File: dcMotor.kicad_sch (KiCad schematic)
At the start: 114 parts, among them J1 USB_C_Receptacle_USB2.0_16P, J2 USB_C_Receptacle_USB2.0_16P, J3 Conn_ST_STDC14, J6 Conn_01x02_Pin, J7 Conn_01x04_Pin, J8 Conn_01x06_Pin, Q1 AO3400A, SW1 SW_Push, SW2 SW_Push, U1 LMR54406DBVR, U10 MCP6561-OT, U2 NCP718ASNADJT1G, U3 NCP718ASNADJT1G, U5 TLV9152IDR, U6 ER_OLEDM0.91_1x-I2C, U7 STM32G431CBTx, U8 LTH-301-05, U9 DRV8231ADDA

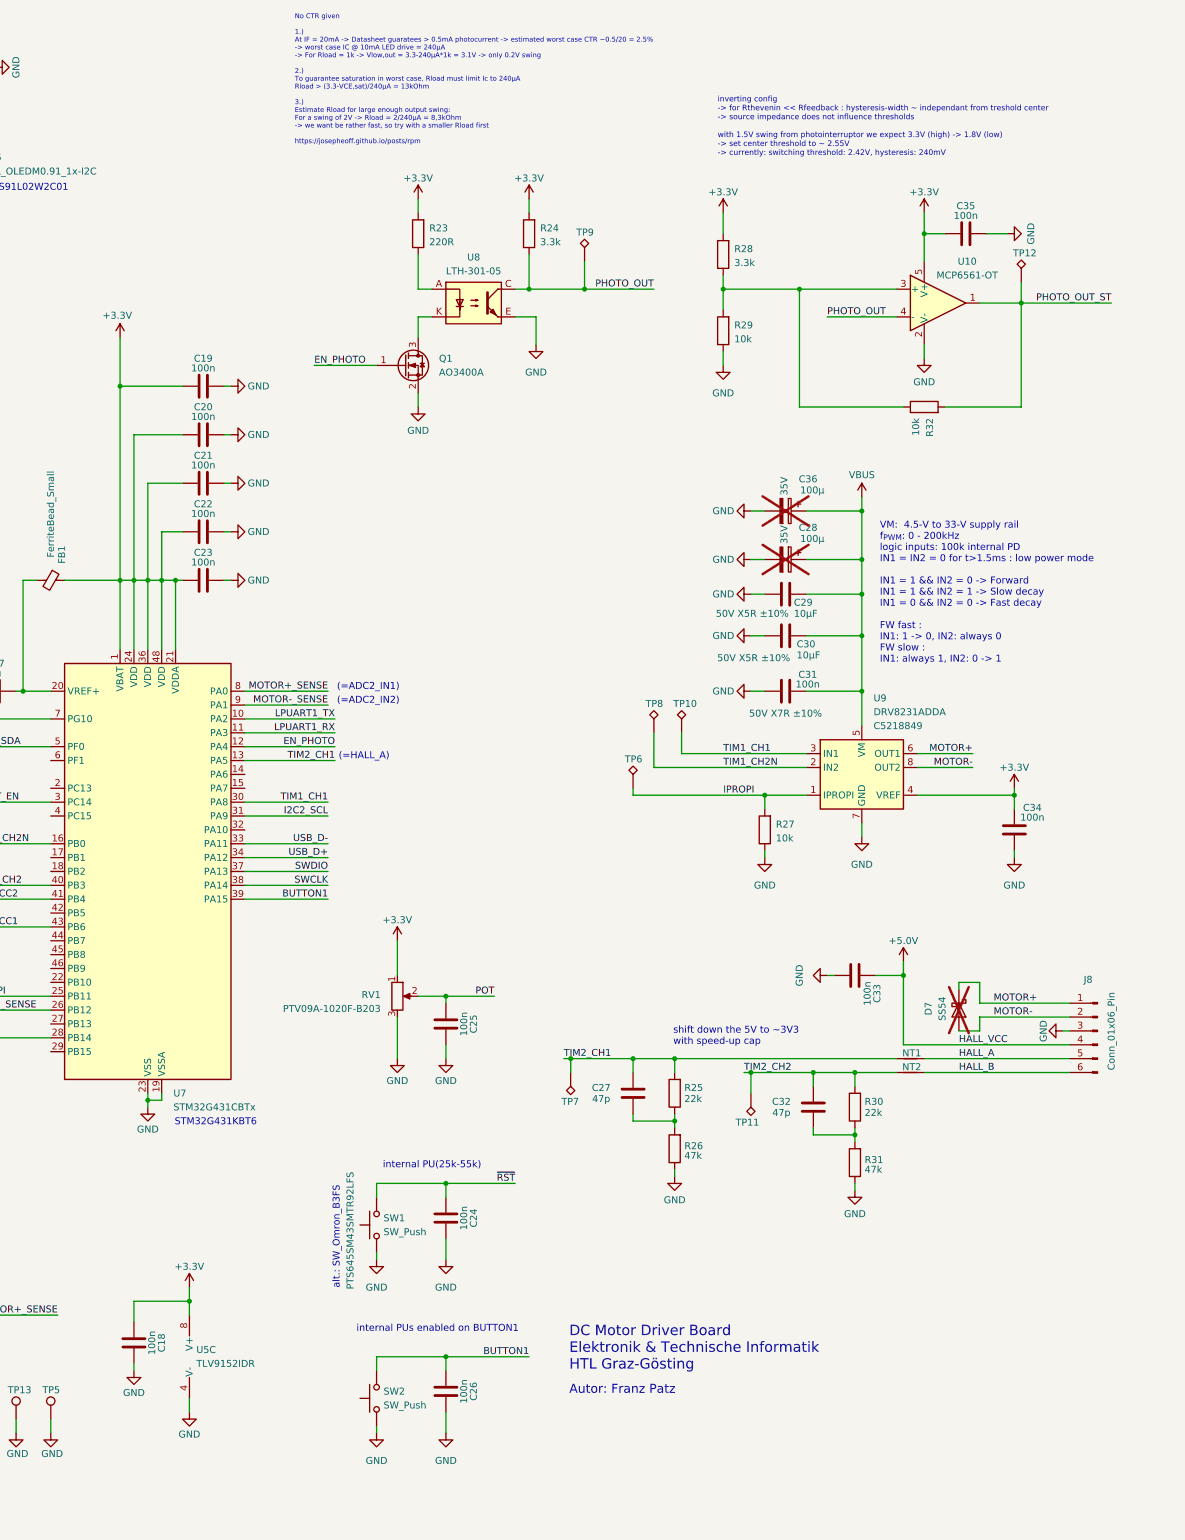
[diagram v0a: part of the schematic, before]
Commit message: finished prel routing
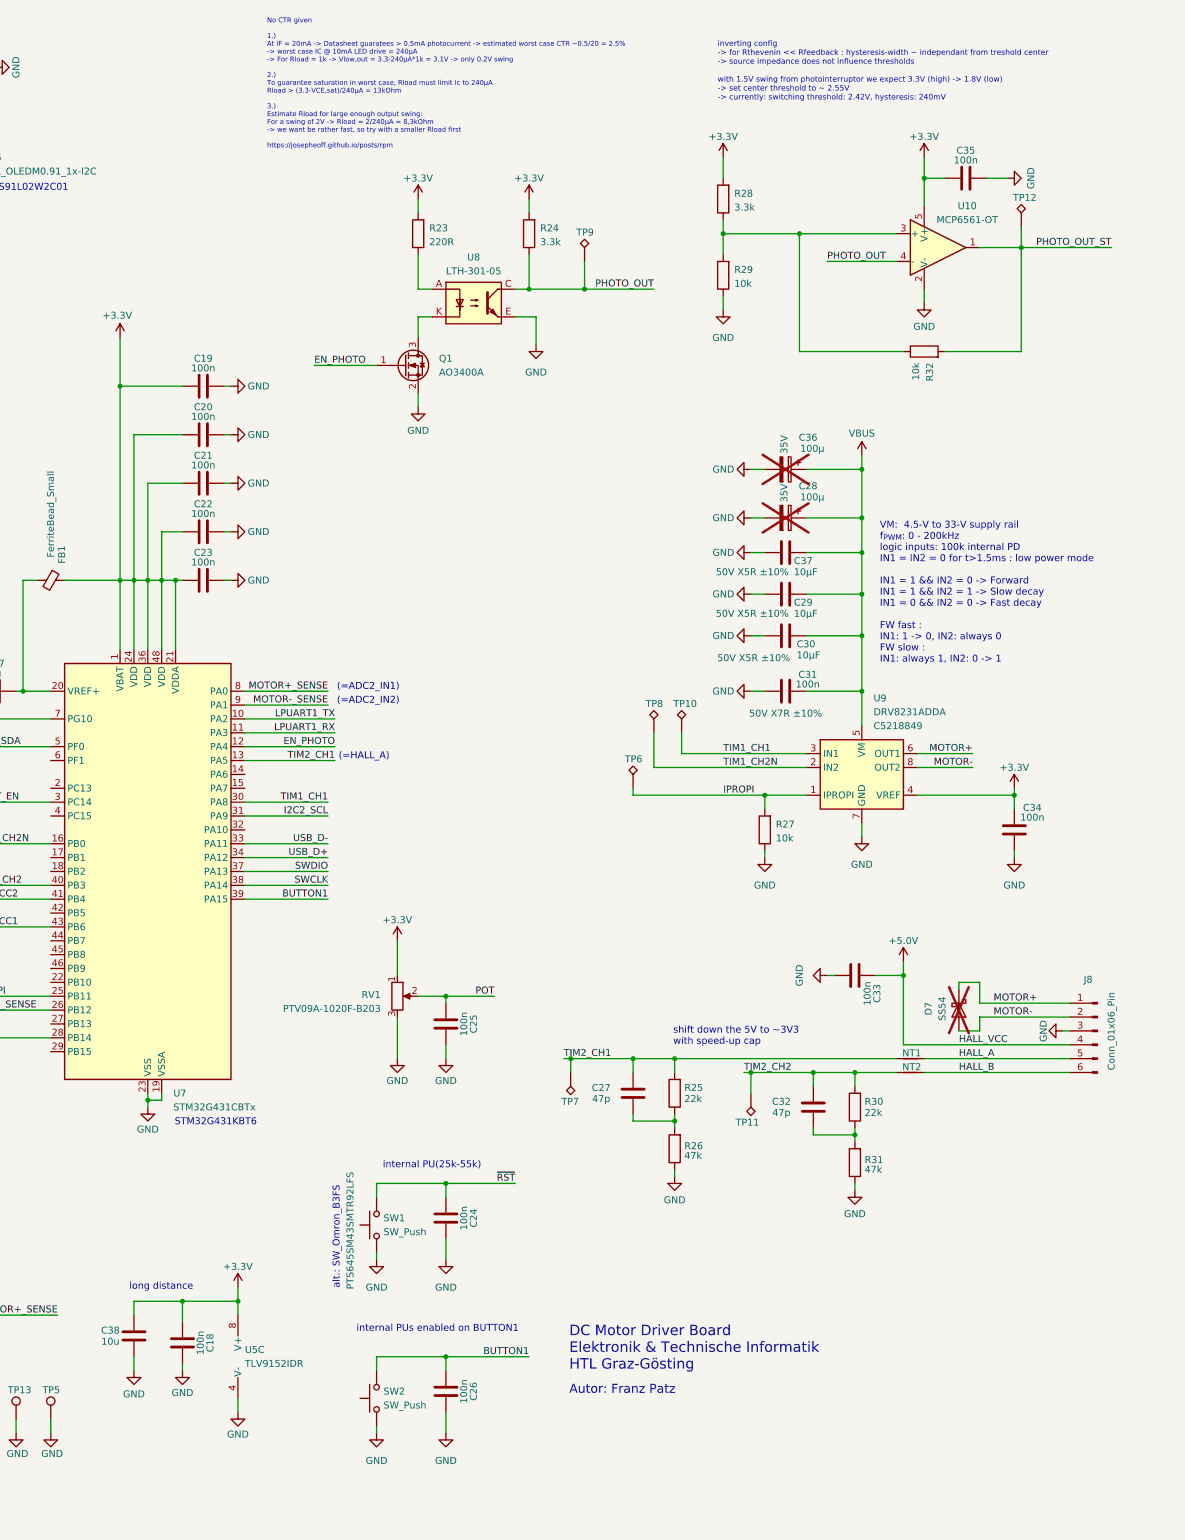
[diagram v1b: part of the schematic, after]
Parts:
- added C37: 10µF, Capacitor_SMD:C_0805_2012Metric_Pad1.18x1.45mm_HandSolder, symbol Device:C
- added C38: 10u, Capacitor_SMD:C_0805_2012Metric, symbol Device:C
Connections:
- net +3.3V: now also C38.2
- net GND: now also C37.2, C38.1
- net VBUS: now also C37.1
- net at U3.4 (ADJ): now also R12.1, R13.2
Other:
- note added: "long distance"
- moved on the sheet: C18, C28, C35, C36, R28, R29, R32, TP12, U10, U5C
